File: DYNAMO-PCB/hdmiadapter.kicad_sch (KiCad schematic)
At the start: 2 parts, among them J1 HDMI_A, U2 CH7035B-BF

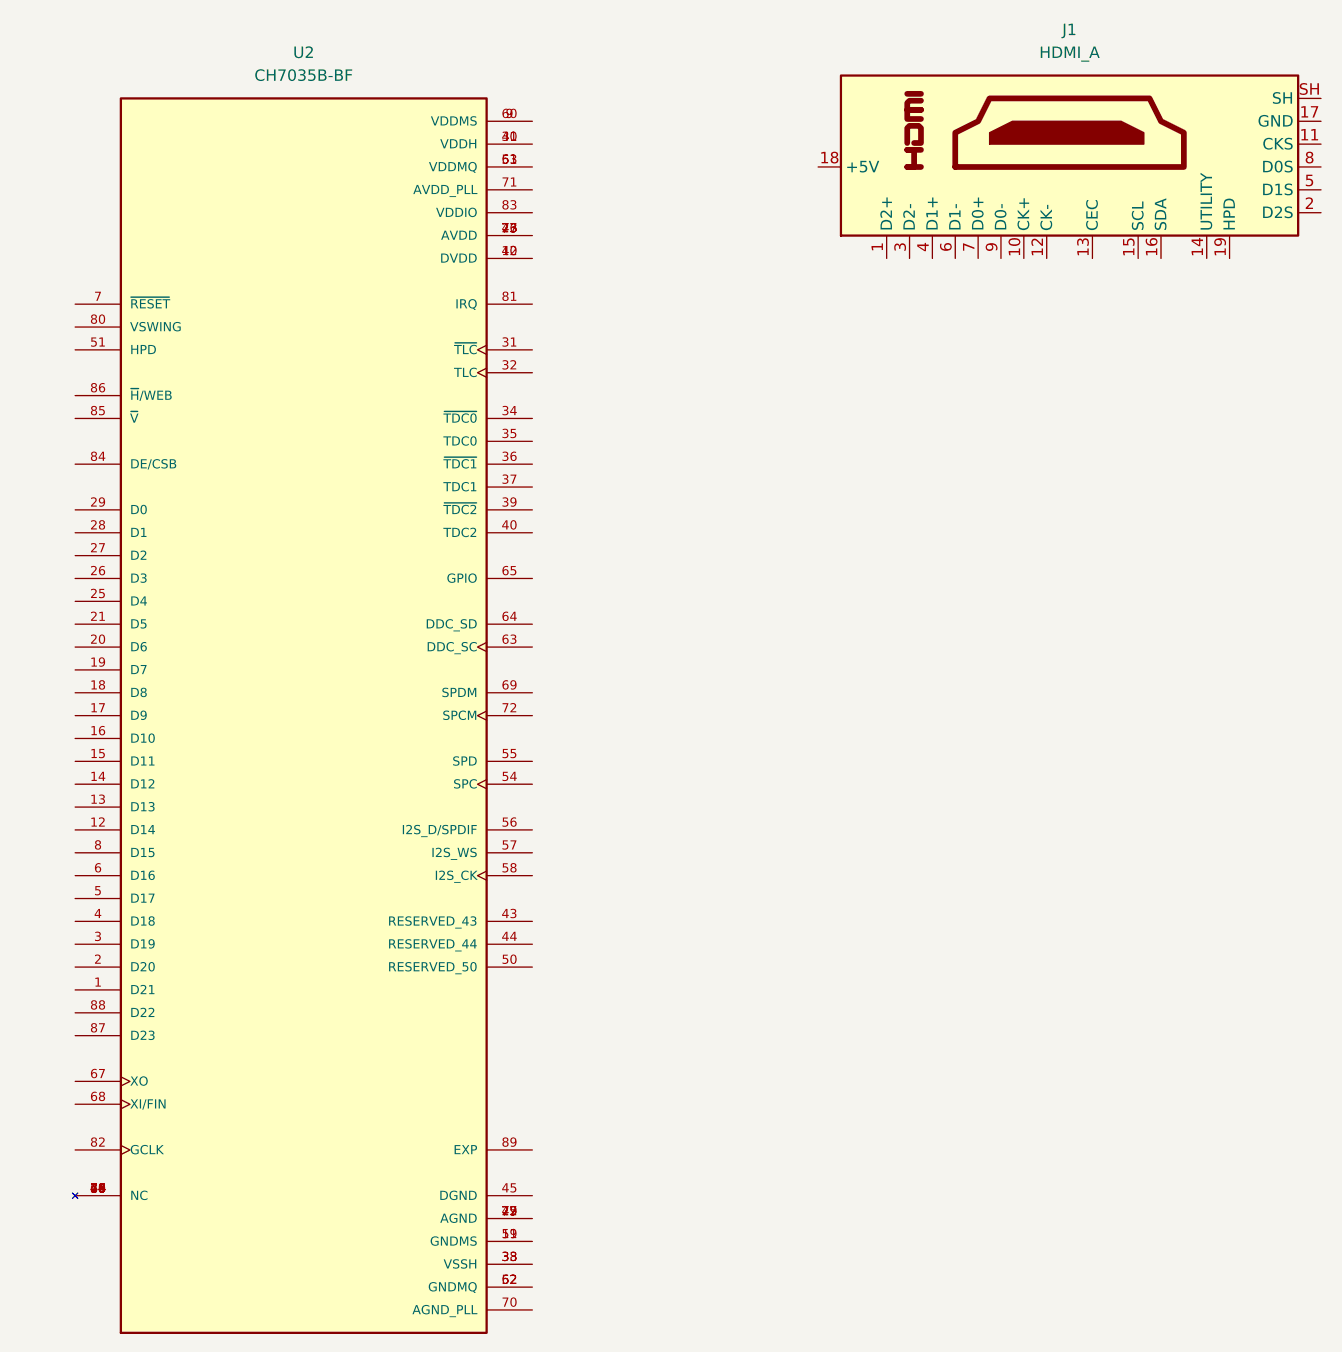
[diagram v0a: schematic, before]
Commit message: schematic wip
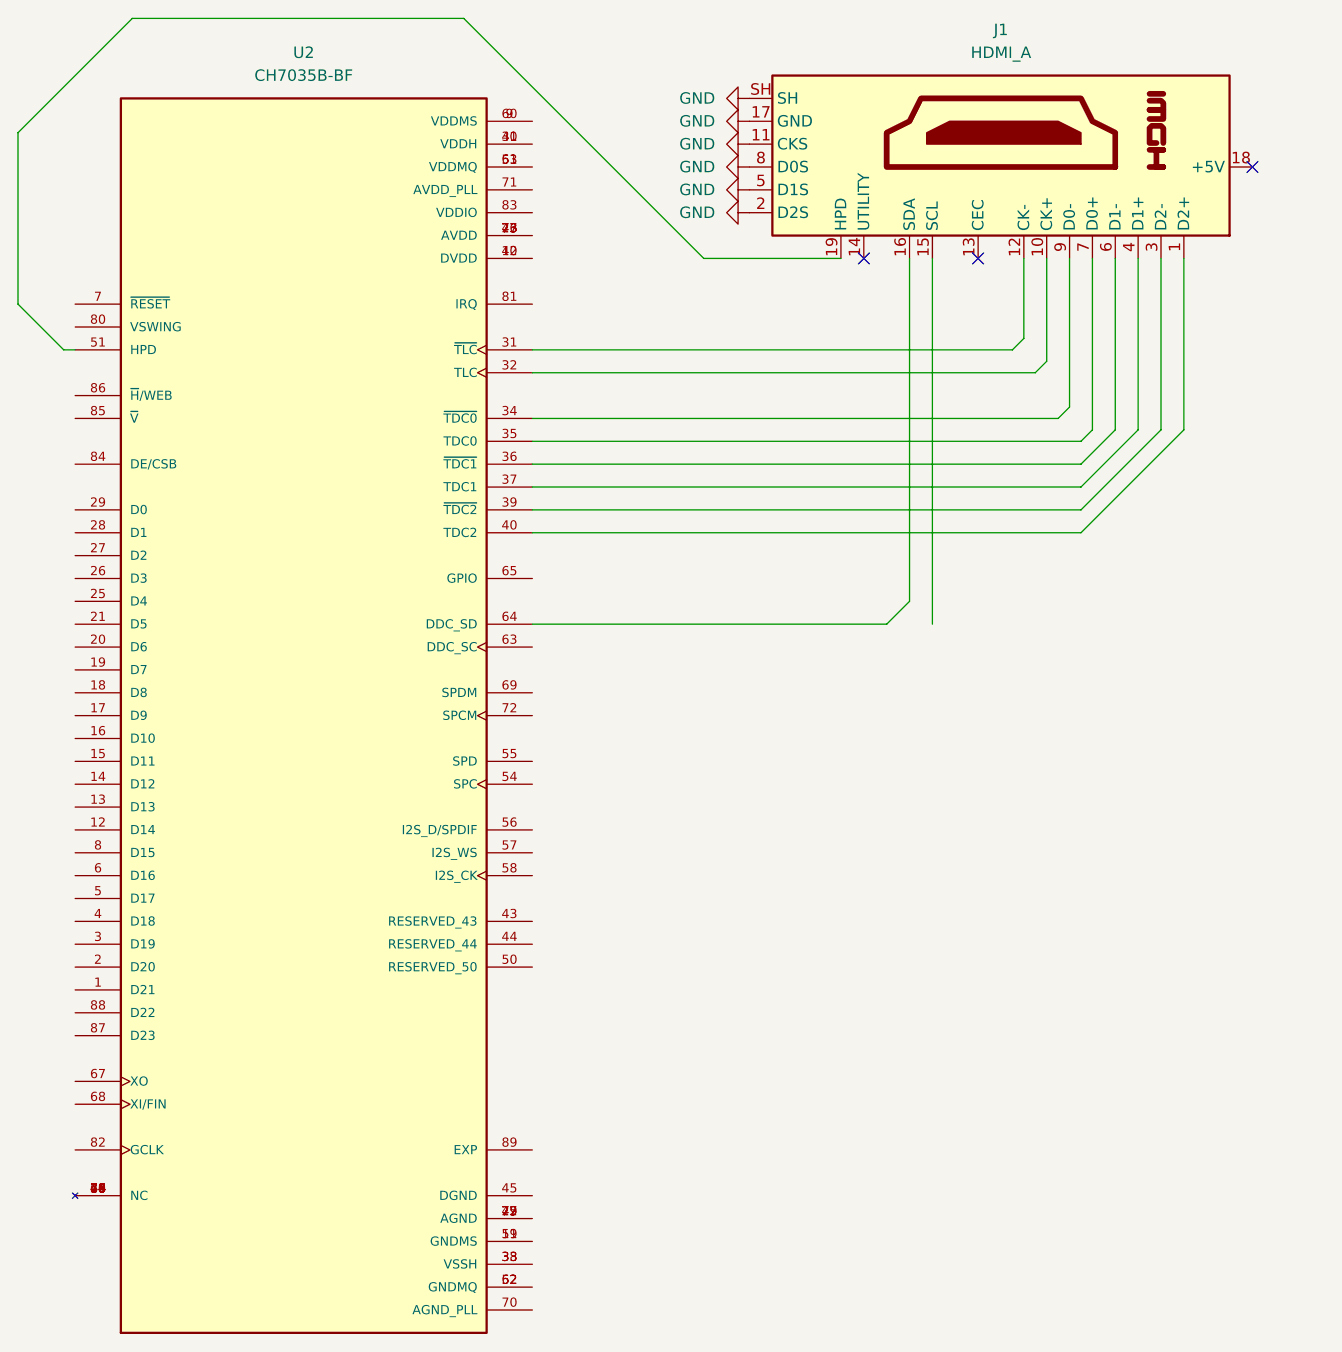
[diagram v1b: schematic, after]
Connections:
- net at U2.31 (~{TLC}): now also J1.12 (CK-)
- net at U2.32 (TLC): now also J1.10 (CK+)
- net at U2.34 (~{TDC0}): now also J1.9 (D0-)
- net at U2.35 (TDC0): now also J1.7 (D0+)
- net at U2.36 (~{TDC1}): now also J1.6 (D1-)
- net at U2.37 (TDC1): now also J1.4 (D1+)
- net at U2.39 (~{TDC2}): now also J1.3 (D2-)
- net at U2.40 (TDC2): now also J1.1 (D2+)
- net at U2.51 (HPD): now also J1.19 (HPD)
- net at U2.64 (DDC_SD): now also J1.16 (SDA)
- net GND: now reaches J1.11 (CKS)
- net GND: now also J1.17 (GND), J1.2 (D2S), J1.5 (D1S), J1.8 (D0S), J1.SH
- no-connect marks 0 -> 3
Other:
- moved on the sheet: J1
